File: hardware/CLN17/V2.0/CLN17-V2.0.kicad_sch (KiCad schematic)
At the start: 78 parts, among them IC1 STM32G431CB, J1 PWR, J10 CAN_OUT, J2 PWR, J3 TYPE-C-31-M-12, J4 Motor, J5 CTRL, J6 CAN, J7 CAN, J8 DEBUG, J9 CAN_IN, SW1 SW_Push, SW2 SW_Push, U1 DRV8844, U10 H5VU25U, U2 TLE5012B, U4 ME6211, U5 H5VU25U, U6 INA180A1, U7 INA180A1, U8 TJA1042, U9 BL9362, Y1 12M

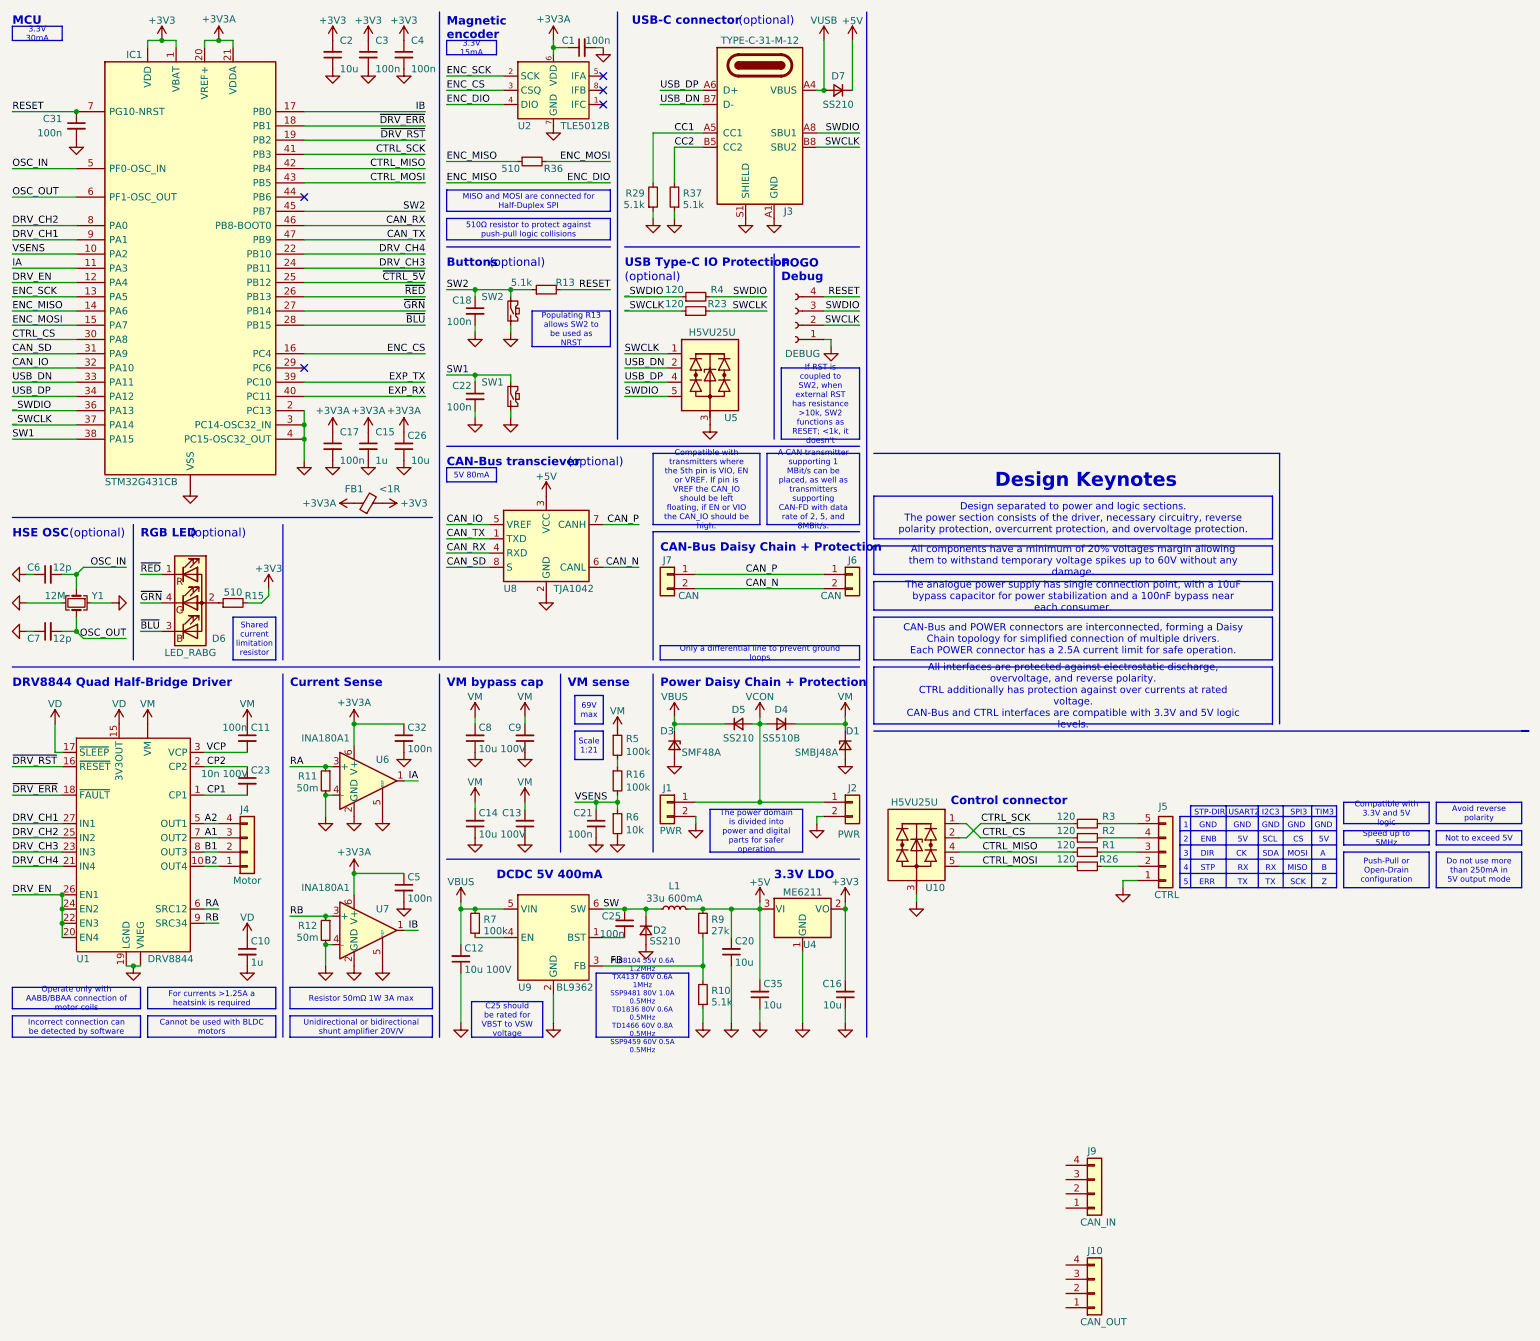
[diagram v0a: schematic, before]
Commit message: [WIP] Before rotating the CAN transceiver
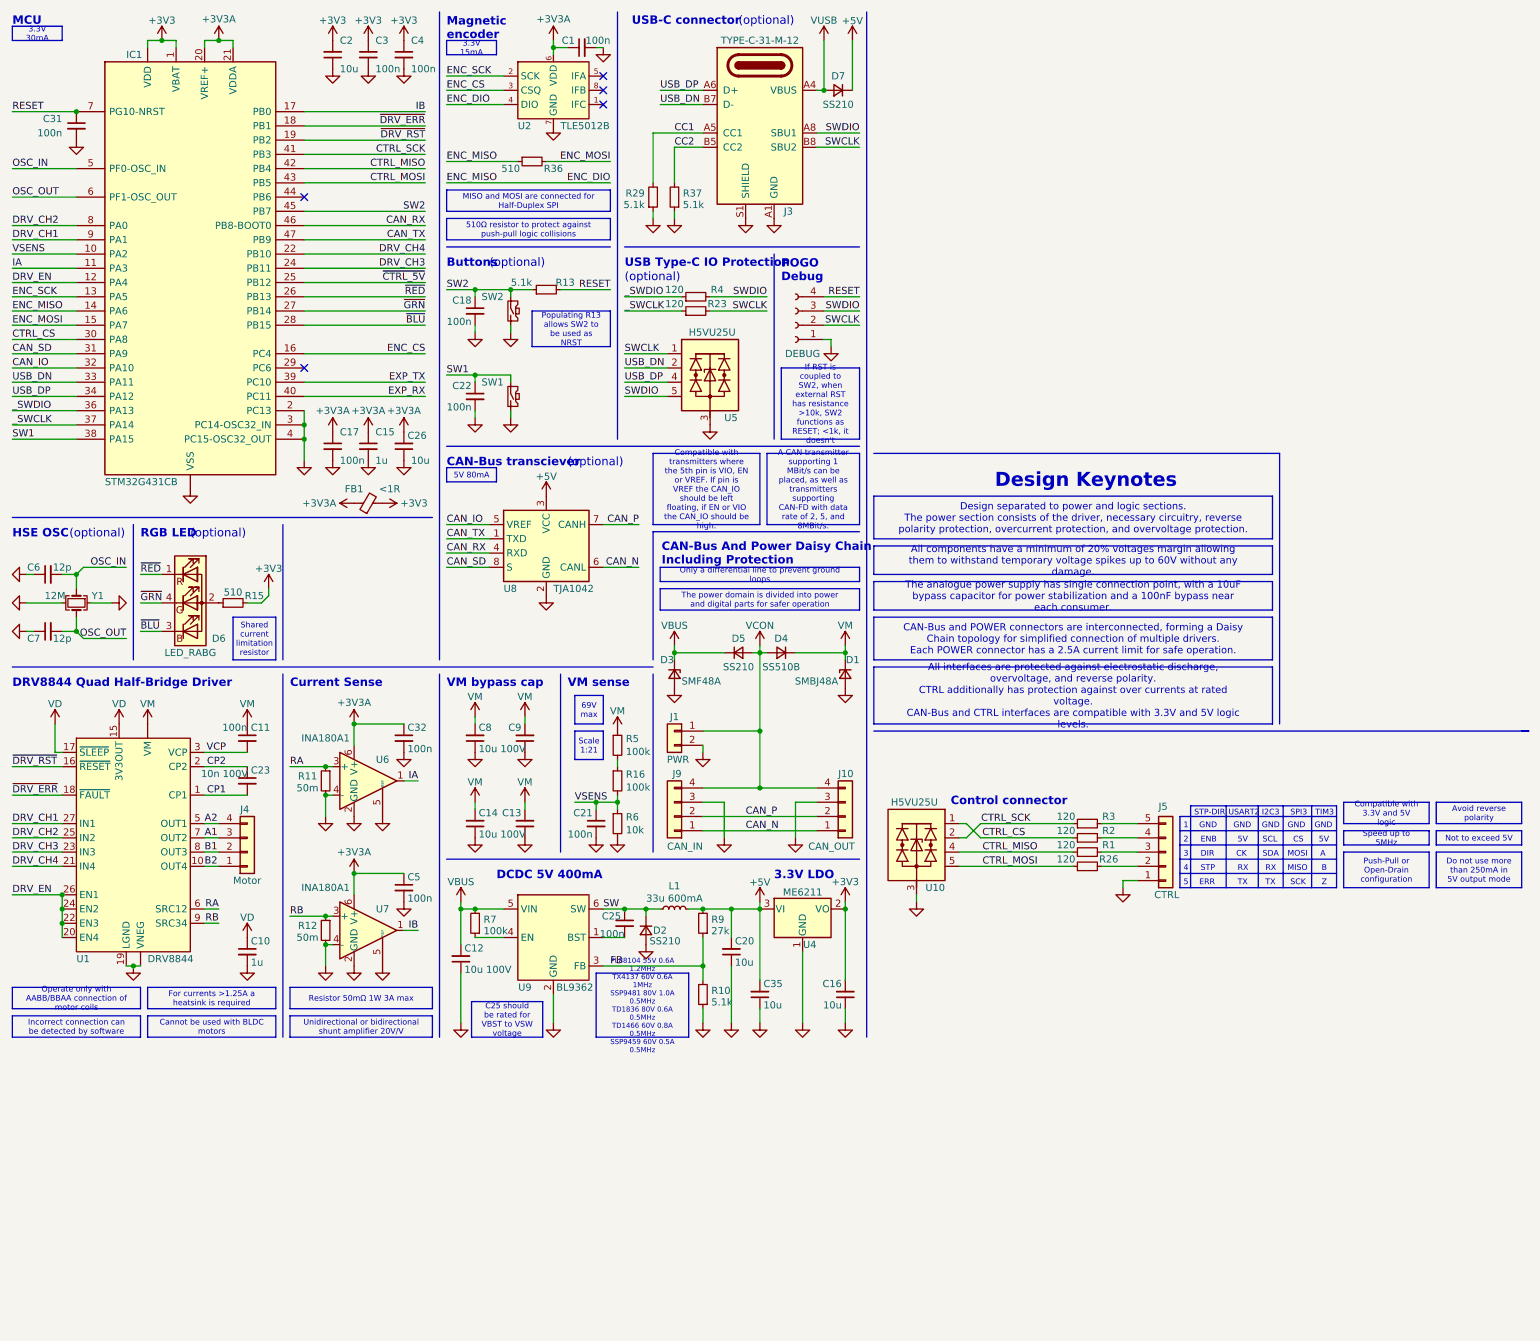
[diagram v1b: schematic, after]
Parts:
- removed J2: PWR, FP_lib:XH2.54 2P, symbol Conn_01x02
- removed J6, J7: CAN, FP_lib:PH2.0 2P, symbol Conn_01x02
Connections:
- net CAN_N: now also J10.1 (Pin_1), J9.1 (Pin_1)
- net CAN_P: now also J10.2 (Pin_2), J9.2 (Pin_2)
- net GND: now also J10.3 (Pin_3), J9.3 (Pin_3)
- net VCON: now also J10.4 (Pin_4), J9.4 (Pin_4)
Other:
- note added: "CAN-Bus And Power Daisy Chain Including Protection"
- note removed: "CAN-Bus Daisy Chain + Protection"
- note removed: "Power Daisy Chain + Protection"
- moved on the sheet: D1, D3, D4, D5, J1, J10, J9
